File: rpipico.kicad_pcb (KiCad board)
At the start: 2 copper layers, 21.2 x 29.1 mm, 35 parts, among them J1 USB_C_Receptacle_USB2.0, J2 Conn_01x02_Pin, J3 Conn_01x13, J4 Conn_01x13, J5 Conn_01x04, J6 Conn_01x03, J7 Conn_01x04, J8 Conn_01x02, J9 Conn_01x02, U2 W25Q128JVS, U3 RP2040, U5 AP2112K-3.3, Y1 12M

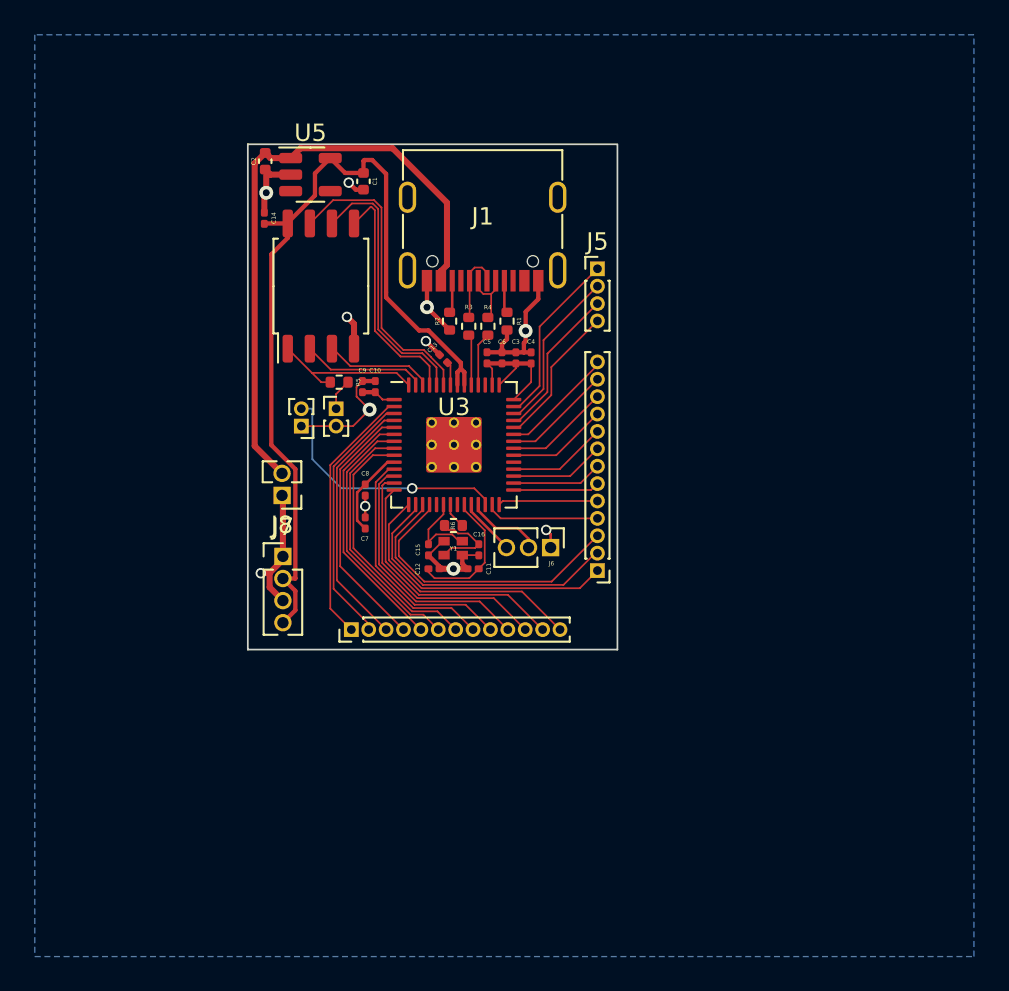
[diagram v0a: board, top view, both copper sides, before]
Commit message: Add files via upload
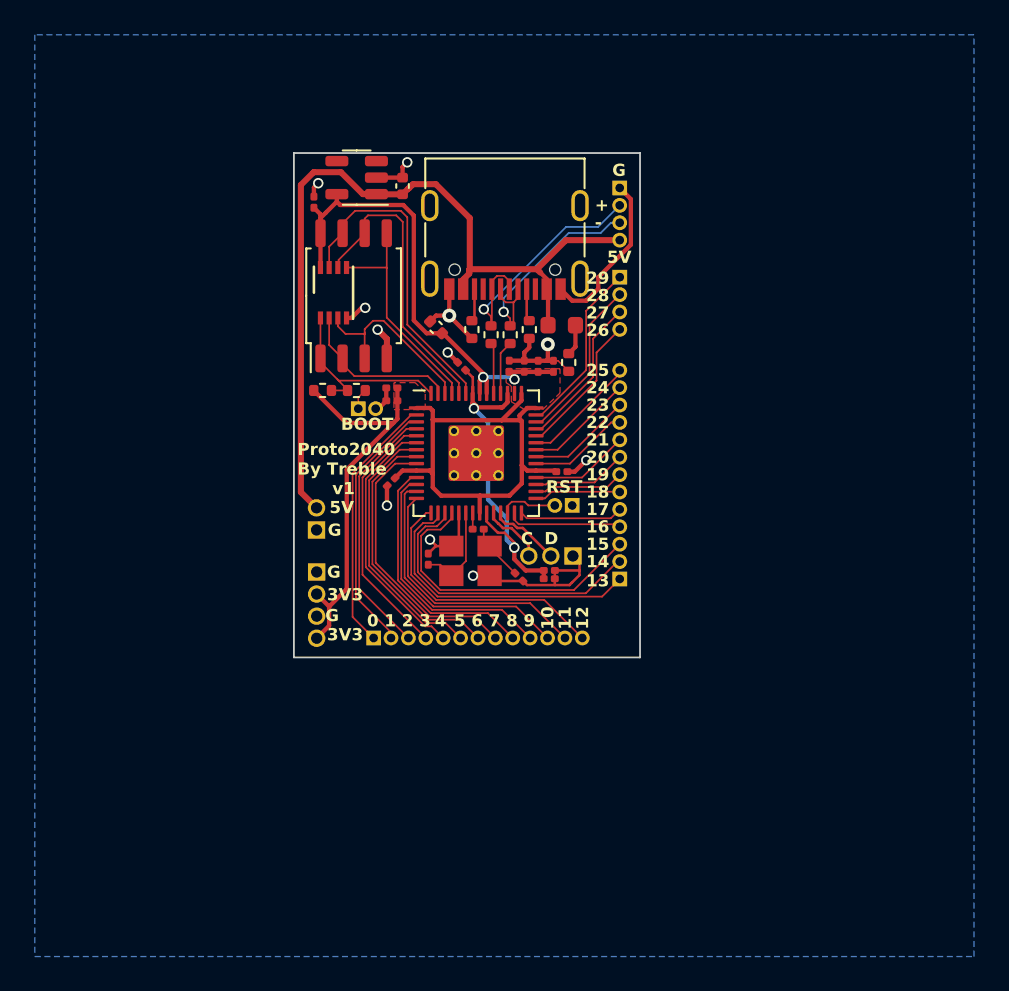
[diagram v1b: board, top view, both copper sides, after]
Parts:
- added D1: LED, LED_SMD:LED_0603_1608Metric, F.Cu at (147.3, 84.7)
- added G***: LOGO, drawings:cute, B.Cu at (138.8, 98.9)
- added J10: Conn_01x04, Connector_PinHeader_1.00mm:PinHeader_1x04_P1.00mm_Vertical, F.Cu at (150.6, 76.8)
- added R8: 10K, Resistor_SMD:R_0402_1005Metric, F.Cu at (133.6, 88.5)
- added R9: 1K, Resistor_SMD:R_0402_1005Metric, F.Cu at (147.7, 86.8)
- added U1: W25Q128JVS, Package_DFN_QFN:DFN-8-1EP_3x2mm_P0.5mm_EP1.3x1.5mm, F.Cu at (134.2, 82.8)
- J2: value Conn_01x02_Pin -> Conn_01x02
- R6: footprint Resistor_SMD:R_0402_1005Metric -> Resistor_SMD:R_0201_0603Metric
- Y1: footprint Crystal2:Crystal_2.0mm_2.5mm -> Crystal:Crystal_SMD_3225-4Pin_3.2x2.5mm
- moved J9 16.2 mm to (147.9, 95.1), turned to -90 degrees
- moved C7 11.7 mm to (147.3, 93.1), turned to 180 degrees
- moved C1 9.38 mm to (140.1, 84.8), turned to 135 degrees
- moved C2 8.02 mm to (138.1, 76.7), turned to 90 degrees
- moved C12 6.63 mm to (146.6, 98.8)
- moved C11 4.41 mm to (146.6, 99.3), turned to 180 degrees
- moved C14 3.00 mm to (133.1, 77.6)
- moved J8 2.80 mm to (133.2, 96.5)
- moved C16 2.79 mm to (144.8, 99.2), turned to -45 degrees
- moved U5 2.66 mm to (135.5, 76.2), turned to 180 degrees
- moved J7 2.14 mm to (133.2, 98.9)
- moved U2 1.96 mm to (135.3, 83.0)
- moved C9 1.88 mm to (137.5, 89.0), turned to 0 degrees
- moved C8 1.56 mm to (137.5, 93.7), turned to 45 degrees
- moved R6 1.44 mm to (142.5, 96.4), turned to 180 degrees
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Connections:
- net D+ renamed /D+
- net D- renamed /D-
- net Net-(J6-Pin_2) renamed /SWD
- net Net-(J6-Pin_3) renamed /SWCLK
- net Net-(J9-Pin_2) renamed /RST
- net Net-(U3-XIN) renamed /XIN
- net Net-(U3-XOUT) renamed /XOUT
- U3 pad 19: unconnected-(U3-TESTEN-Pad19) -> GND
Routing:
- net +3.3V: track 66.6 -> 80.0 mm, vias 0 -> 2
- net +1V1: track 9.13 -> 22.2 mm, vias 0 -> 2
- net VBUS: track 36.3 -> 48.0 mm
- net /D+: track 4.31 -> 15.7 mm, vias 0 -> 1
- net /RST: track 14.7 -> 3.31 mm, vias 1 -> 0
- net /D-: track 4.18 -> 14.4 mm, vias 0 -> 1
- net /QSPI_SD2: track 6.26 -> 10.8 mm
- net GND: track 42.2 -> 45.9 mm
- net /QSPI_SS: track 9.16 -> 11.8 mm
- net /QSPI_SD1: track 7.13 -> 9.40 mm
- net Net-(D1-K): track 0.00 -> 1.79 mm
- net Net-(C16-Pad1): track 4.67 -> 3.27 mm
- net /QSPI_CLK: track 16.1 -> 17.1 mm
- net /QSPI_SD3: track 17.9 -> 18.6 mm
- net Net-(J4-Pin_3): track 16.8 -> 17.5 mm
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- added copper zone on F.Cu, net +3.3V
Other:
- board size 21.2 x 29.1 mm -> 19.9 x 29 mm
- board text added: "+"
- board text added: "-"
- board text added: "0"
- board text added: "1"
- board text added: "10"
- board text added: "11"
- board text added: "12"
- board text added: "13"
- board text added: "14"
- board text added: "15"
- board text added: "16"
- board text added: "17"
- board text added: "18"
- board text added: "19"
- board text added: "2"
- board text added: "20"
- board text added: "21"
- board text added: "22"
- board text added: "23"
- board text added: "24"
- board text added: "25"
- board text added: "26"
- board text added: "27"
- board text added: "28"
- board text added: "29"
- board text added: "3"
- board text added: "3V3"
- board text added: "4"
- board text added: "5"
- board text added: "5V"
- board text added: "6"
- board text added: "7"
- board text added: "8"
- board text added: "9"
- board text added: "BOOT"
- board text added: "C"
- board text added: "D"
- board text added: "G"
- board text added: "Proto2040 By Treble v1"
- board text added: "RST"
